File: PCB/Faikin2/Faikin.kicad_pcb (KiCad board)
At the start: 2 copper layers, 70 x 70 mm, 25 parts, among them J1 1x5, J2 Shelly, J3 USB-PROG, Q1 BSS138PS, U3 MD8942, U4 ESP32-S3-MINI-1

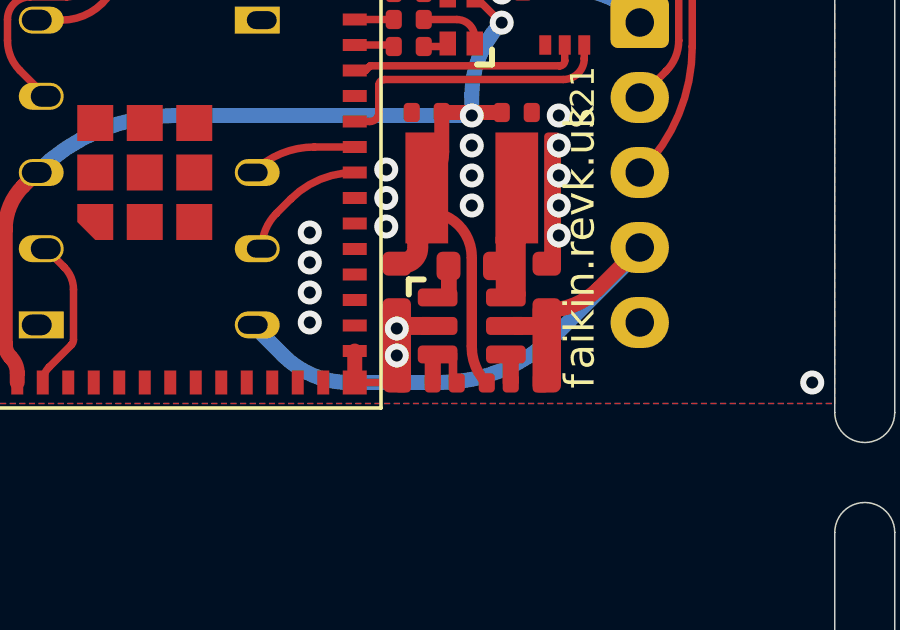
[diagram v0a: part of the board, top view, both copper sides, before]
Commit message: More tidy
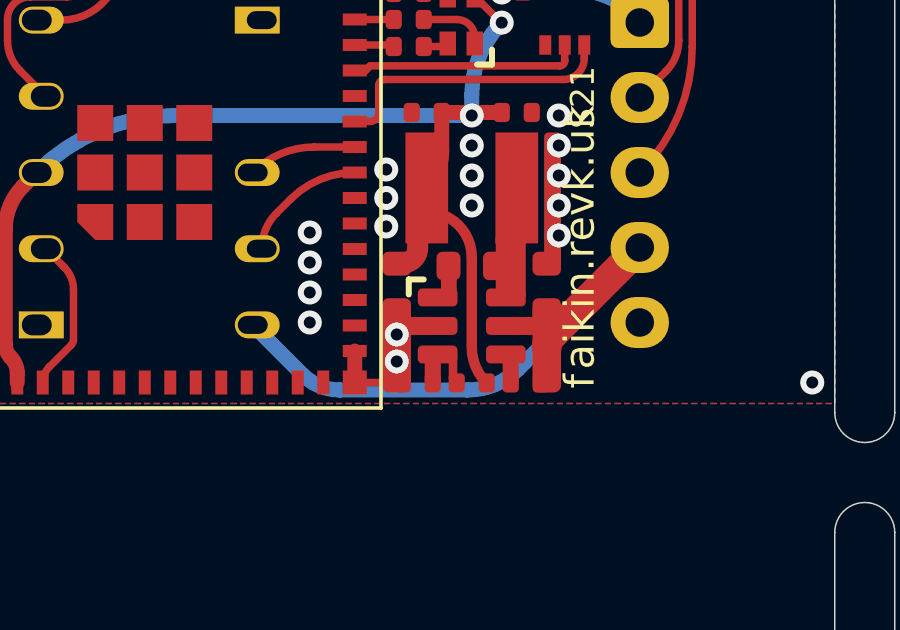
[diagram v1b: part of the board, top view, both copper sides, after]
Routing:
- net DC: track 18.9 -> 20.2 mm
